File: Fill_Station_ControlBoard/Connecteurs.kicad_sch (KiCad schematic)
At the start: 34 parts, among them J6 RJ45_Wuerth_7499010211A, U5 LAN8742A

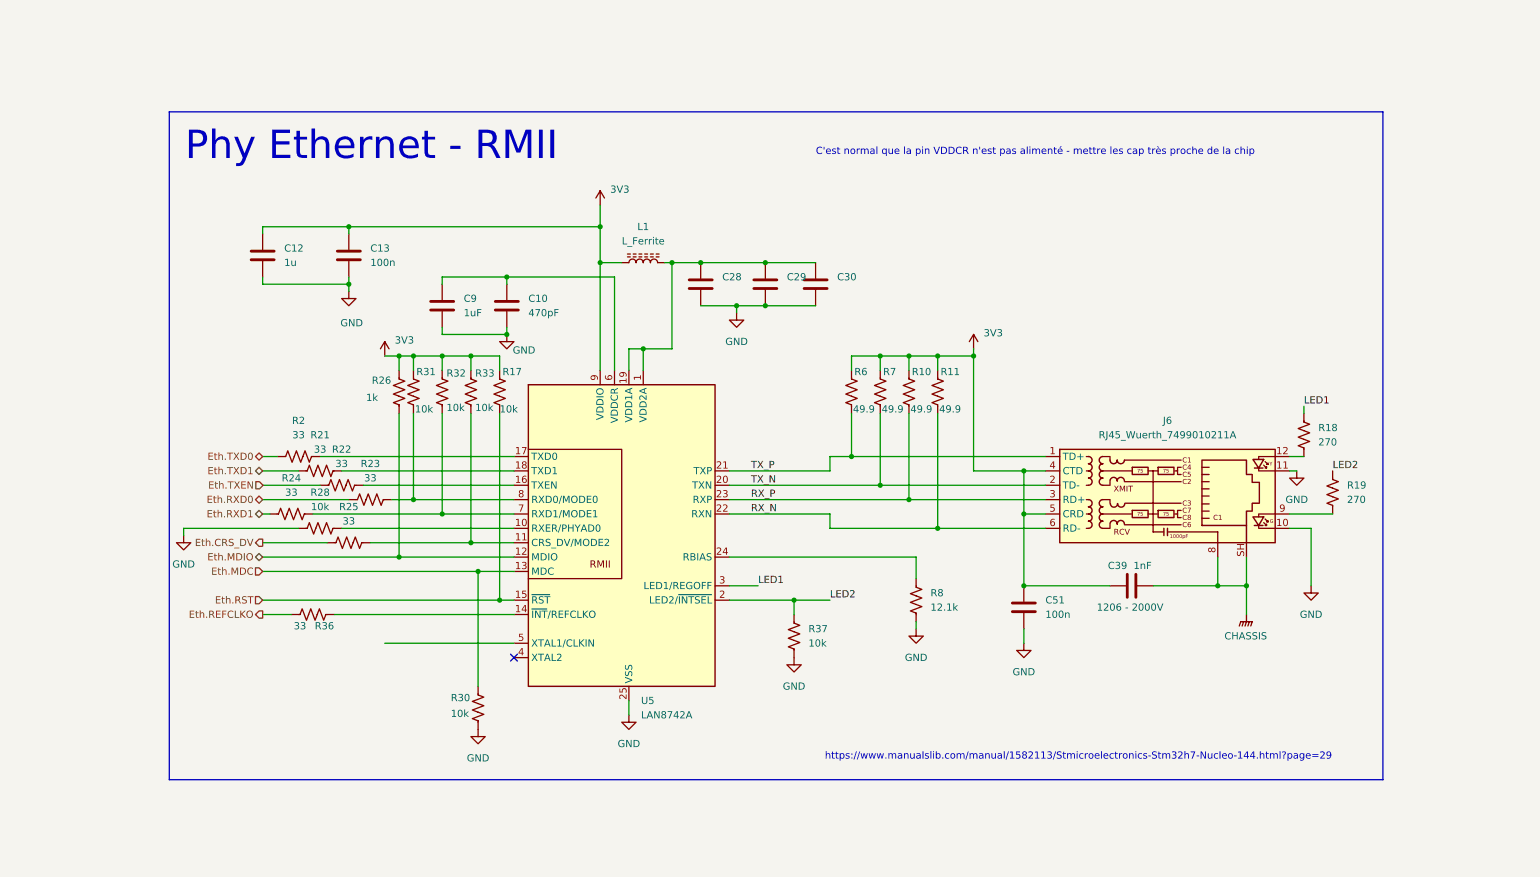
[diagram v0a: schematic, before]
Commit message: début layout
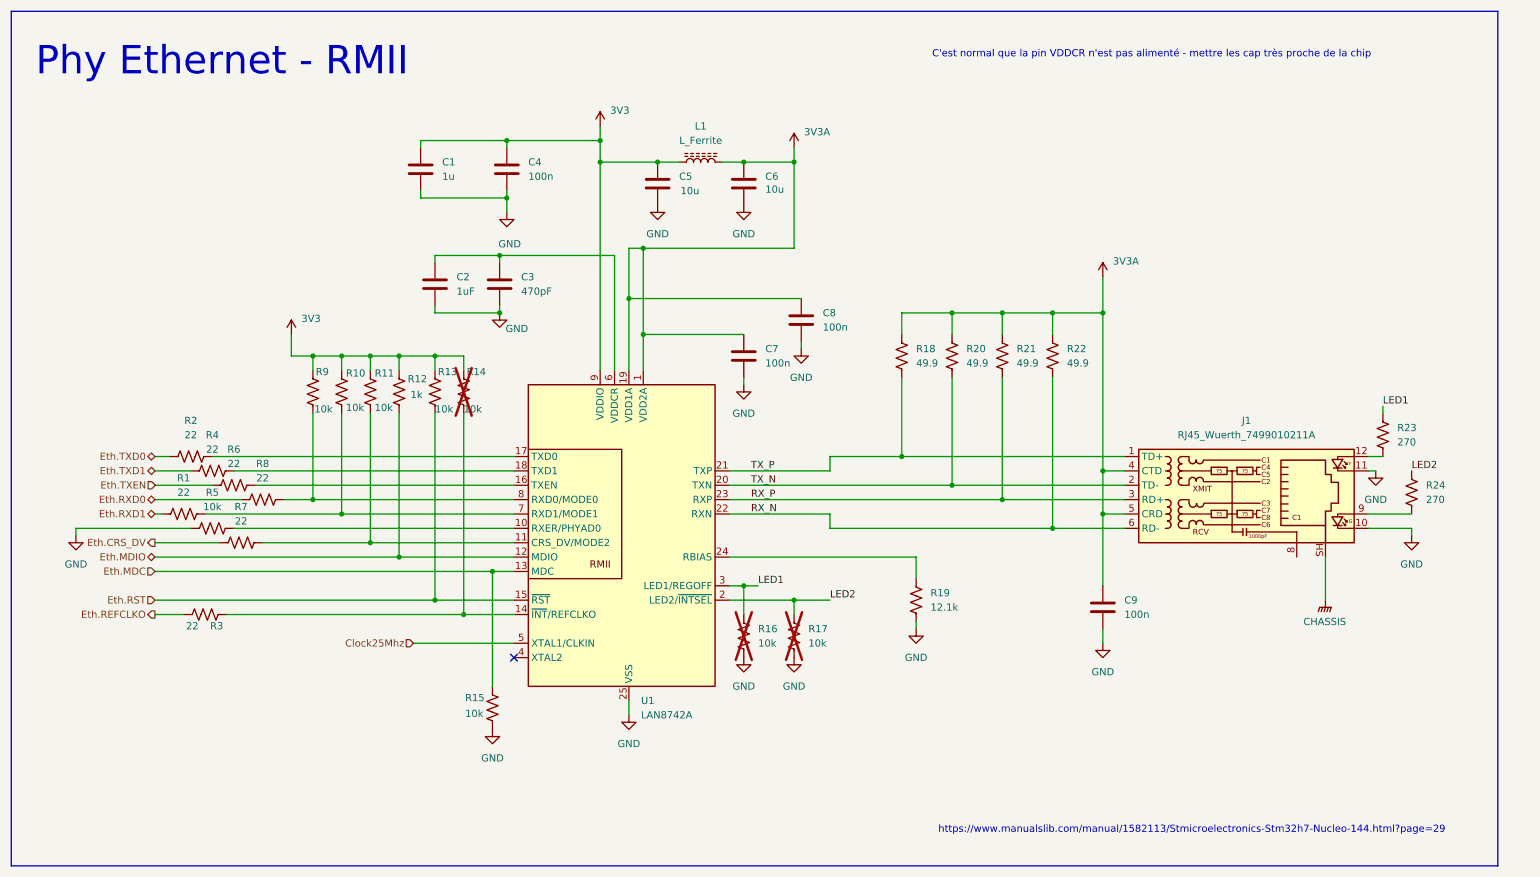
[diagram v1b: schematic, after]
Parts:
- removed C30: ~, Capacitor_SMD:C_0603_1608Metric, symbol Device:C
- removed C39: 1nF, Capacitor_SMD:C_0603_1608Metric, symbol Device:C
- removed R10, R11: 49.9, Capacitor_SMD:C_0603_1608Metric, symbol Device:R_US
- removed R6, R7: 49.9, Resistor_SMD:R_0603_1608Metric_Pad0.98x0.95mm_HandSolder, symbol Device:R_US
- added C5: 10u, Capacitor_SMD:C_0603_1608Metric, symbol Device:C
- added C8: 100n, Capacitor_SMD:C_0603_1608Metric, symbol Device:C
- added R14, R16: 10k, Resistor_SMD:R_0603_1608Metric_Pad0.98x0.95mm_HandSolder, symbol Device:R_US
- added R18, R20, R21, R22: 49.9, Resistor_SMD:R_0603_1608Metric_Pad0.98x0.95mm_HandSolder, symbol Device:R_US
- C6: renamed from C28; value ~ -> 10u
- C7: renamed from C29; value ~ -> 100n
- R1: renamed from R24; value 33 -> 22
- R17: renamed from R37; now not fitted
- R2: value 33 -> 22
- R3: renamed from R36; value 33 -> 22
- R4: renamed from R21; value 33 -> 22
- R6: renamed from R22; value 33 -> 22
- R7: renamed from R25; value 33 -> 22
- R8: renamed from R23; value 33 -> 22
- renumbered C12 to C1, C9 to C2, C10 to C3, C13 to C4, C51 to C9, J6 to J1, R32 to R10, R33 to R11, R26 to R12, R17 to R13, R30 to R15, R8 to R19, R18 to R23, R19 to R24, R28 to R5, R31 to R9, U5 to U1
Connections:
- net 3V3: now also C5.1, R14.1; no longer C9.1, J1.4 (CTD), J1.5 (CRD)
- net CHASSIS: no longer J1.8
- net GND: now also C5.2, C8.2, R16.2
- net LED1: now also R16.1
- net RX_N: now also R22.2
- net RX_P: now also R21.2
- net TX_N: now also R20.2
- net TX_P: now also R18.2
- net at R3.2, U1.14 (~{INT}/REFCLKO): now also R14.2
- net 3V3A: now reaches C6.1, C7.1, L1.2, U1.1 (VDD2A), U1.19 (VDD1A)
- net 3V3A: now also C9.1, J1.4 (CTD), J1.5 (CRD), C8.1, R18.1, R20.1, R21.1, R22.1
- net Clock25Mhz: now reaches U1.5 (XTAL1/CLKIN)
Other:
- moved on the sheet: C1, C2, C3, C4, C6, C7, C9, J1, L1, R1, R10, R11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
